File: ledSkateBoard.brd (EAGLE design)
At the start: 23 x 47.6 mm, 25 parts, among them J1 JST, U1 MPU-9150, U2 ATMEGA328P_TQFP, U4 MIC2505 3.3

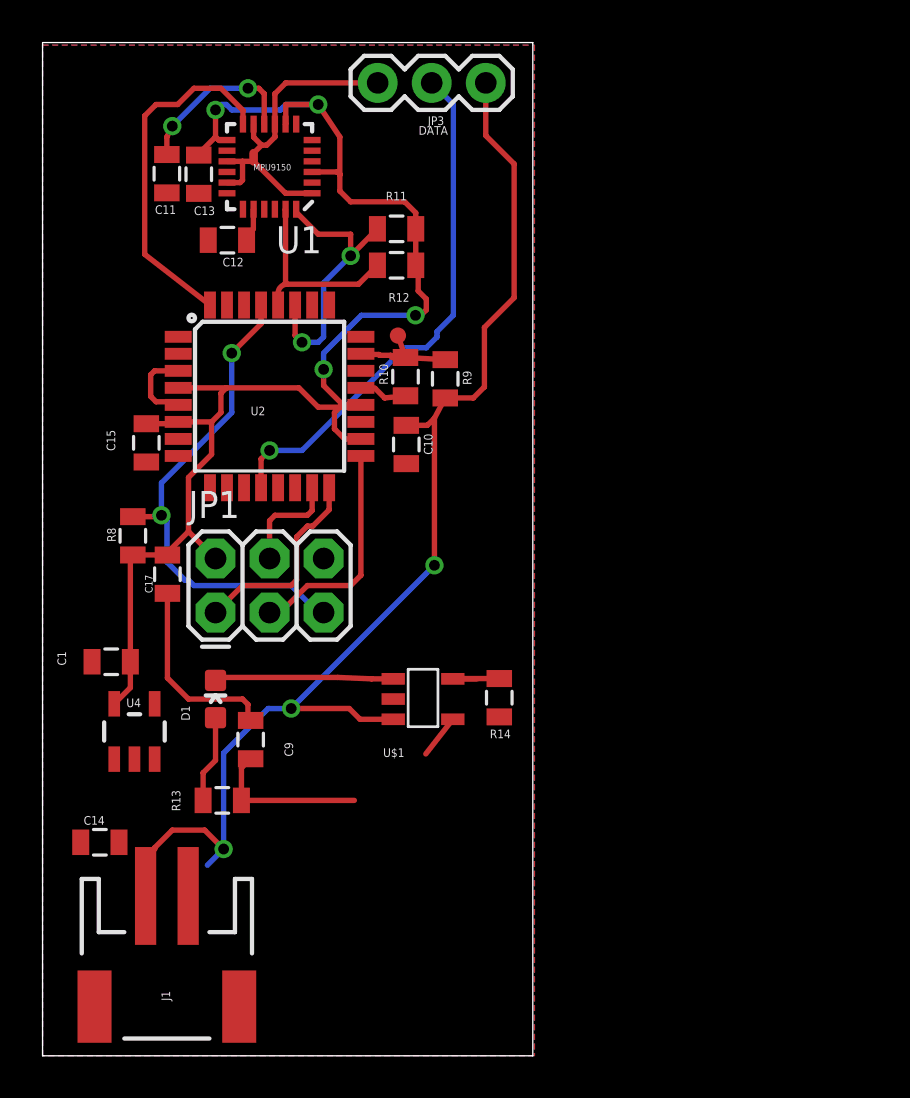
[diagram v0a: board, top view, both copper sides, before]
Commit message: Final on revA
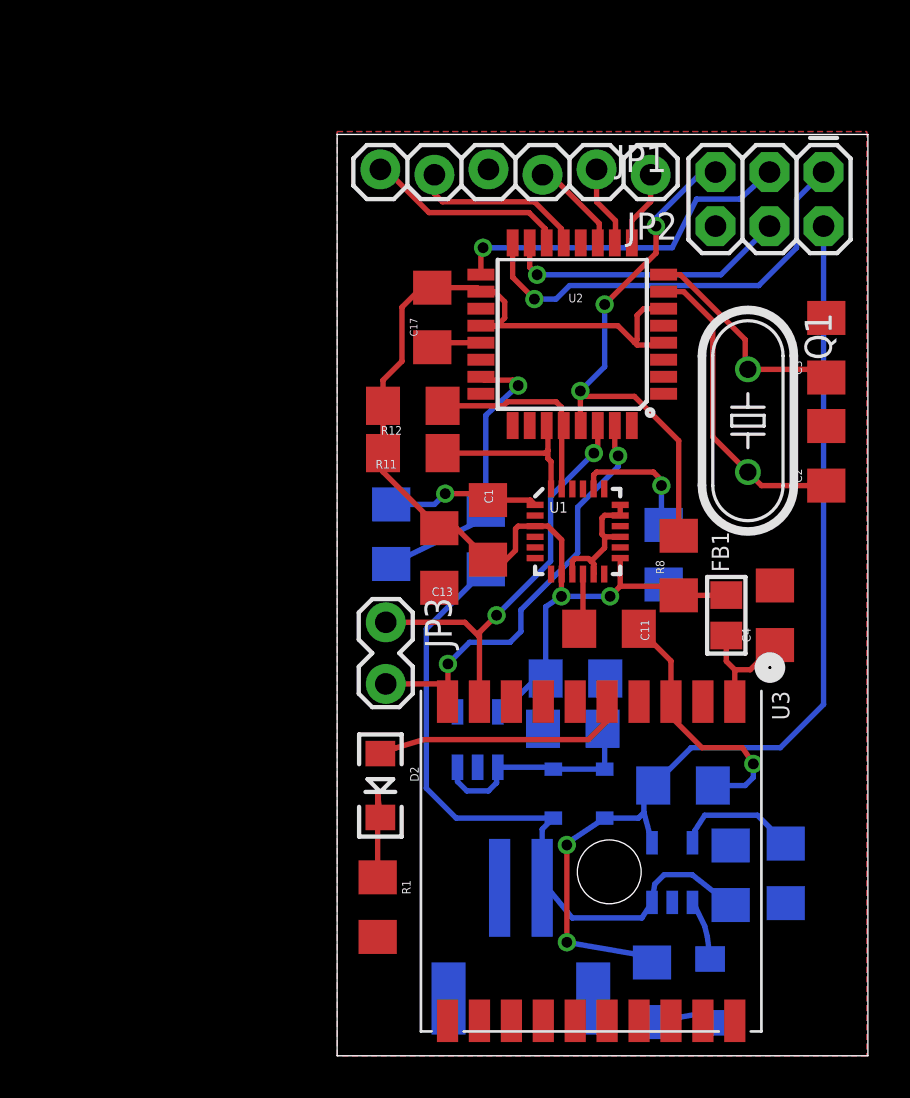
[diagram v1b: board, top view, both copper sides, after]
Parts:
- removed R10: 36K, SparkFun-Resistors:0805
- removed R9: 4.3K, SparkFun-Resistors:0805
- removed TP3: TEST-POINT3, SparkFun-Passives:PAD.03X.03
- added C2, C3: 22pF, SparkFun-Capacitors:1206
- added C4: 10uF, SparkFun-Capacitors:1206
- added D2: GREEN, SparkFun-LED:LED-1206
- added D3, D4: PMEG4005EJ, SparkFun-DiscreteSemi:SOD-323
- added FB1: (no value), microbuilder:0805
- added JP2: (no value), SparkFun-Connectors:1X06_LOCK
- added Q1: 16Mhz, adafruit:HC49/S
- added R1: 330, SparkFun-Passives:1206
- added R2: 37K, SparkFun-Passives:1206
- added R3: 430K, SparkFun-Passives:1206
- added U3: (no value), adafruit:FGPMMOPA6H
- C1: value 10uF -> 10nF; device SparkFun-Capacitors:0805 -> SparkFun-Capacitors:1206
- C10, C13, C14, C15, C17, C9: device SparkFun-Capacitors:0805 -> SparkFun-Capacitors:1206
- C11: value 4.7uF -> .1uF; device SparkFun-Capacitors:0805 -> SparkFun-Capacitors:1206
- C12: value 4.7uF -> 2.2nF 50V; device SparkFun-Capacitors:0805 -> SparkFun-Capacitors:1206
- D1: device SparkFun-LED:LED-0603 -> SparkFun-LED:LED-1206
- JP3: value LED CONNECTOR -> M02LOCK; device SparkFun-Connectors:1X03 -> SparkFun-Connectors:1X02_LOCK
- R11, R12: value 10K -> 4.7K; device SparkFun-Resistors:0805 -> SparkFun-Passives:1206
- R13, R14, R8: device SparkFun-Resistors:0805 -> SparkFun-Passives:1206
- moved JP1 35.3 mm to (66.7, 41.0), turned to 180 degrees
- moved C11 29.8 mm to (56.6, 19.6), turned to 0 degrees
- moved D1 27.0 mm to (61.3, 2.54), flipped to the bottom, turned to 90 degrees
- moved JP3 26.0 mm to (46.1, 19.7), turned to 270 degrees
- moved R8 25.7 mm to (59.9, 22.5)
- moved C10 25.3 mm to (62.3, 7.98), flipped to the bottom, turned to 90 degrees
- moved C12 25.3 mm to (59.2, 23.0), flipped to the bottom, turned to 270 degrees
- moved C15 23.0 mm to (55.0, 17.2), flipped to the bottom, turned to 0 degrees
- moved C14 22.9 mm to (54.9, 14.9), flipped to the bottom, turned to 180 degrees
- moved U1 22.4 mm to (55.1, 24.1), turned to 0 degrees
- moved R13 22.1 mm to (58.6, 2.48), flipped to the bottom, turned to 90 degrees
- moved C13 21.3 mm to (48.6, 22.9)
- moved C9 20.4 mm to (60.1, 12.2), flipped to the bottom, turned to 180 degrees
- moved C1 18.8 mm to (50.9, 24.2), turned to 270 degrees
- moved C17 17.3 mm to (48.3, 34.2)
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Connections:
- removed net DATA: JP3.2, U2.12
- removed net MPU_INT: U1.12, U2.32
- new net AN0: JP2.2, U2.10
- new net AN1: JP2.3, U2.11
- new net GPS_RX: JP3.2, U2.31, U3.P$10
- new net GPS_TX: JP3.1, U2.30, U3.P$9
- new net N$10: C14.2, D3.C, D4.C, U4.1, U4.3
- new net N$3: C2.1, Q1.2, U2.7
- new net N$5: C3.1, Q1.1, U2.8
- new net N$6: D2.A, U3.P$5
- new net N$9: D2.C, R1.1
- new net PB0: JP2.4
- new net PB1: JP2.5, U2.13
- new net PB2: JP2.6, U2.14
- new net PD5: JP2.1, U2.9
- new net PWR_MNTR: R2.1, R3.2, U2.23
- net 5V: now also D3.A, JP1.2
- net GND: now also C2.2, C3.2, C4.2, R1.2, R3.1, U3.P$19, U3.P$3, U3.P$8; no longer JP3.3, R10.1
- net N$4: now also C4.1, FB1.1, U3.P$1; no longer R10.2, R9.1, TP3.P$1, U2.23
- net VCC: now also FB1.2; no longer JP1.2
- net V_BATT: now also D4.A, R2.2; no longer C14.2, JP3.1, R9.2, U4.1, U4.3
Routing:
- net 5V: track 9.51 -> 48.1 mm, vias 0 -> 2
- net DATA: track 24.7 -> 0.00 mm, vias 1 -> 0
- net V_BATT: track 57.5 -> 32.8 mm, vias 3 -> 0
- net GPS_RX: track 0.00 -> 20.5 mm, vias 0 -> 2
- net GPS_TX: track 0.00 -> 20.0 mm, vias 0 -> 2
- net MPU_INT: track 16.6 -> 0.00 mm
- net N$3: track 0.00 -> 14.6 mm
- net PWR_MNTR: track 0.00 -> 13.8 mm, vias 0 -> 1
- net N$6: track 0.00 -> 12.5 mm
- net MISO: track 9.57 -> 20.5 mm, vias 0 -> 1
- net VCC: track 68.9 -> 58.3 mm, vias 4 -> 2
- net N$10: track 0.00 -> 10.6 mm
- net N$5: track 0.00 -> 10.4 mm
- net PB2: track 0.00 -> 9.59 mm
- net MOSI: track 5.05 -> 13.5 mm, vias 0 -> 1
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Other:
- board size 23 x 47.6 mm -> 24.9 x 43.3 mm
- board text removed: "DATA"
- board text removed: "MPU9150"
